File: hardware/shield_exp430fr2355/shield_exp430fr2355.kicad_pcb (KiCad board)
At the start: 2 copper layers, 74.6 x 50 mm, 50 parts, among them J1 TI_BOOSTER_40_J1, J10 Conn_01x02_Male, J12 Conn_01x02_Male, J13 Conn_01x02_Male, J14 Conn_01x02_Male, J15 Conn_01x02_Male, J16 Conn_01x02_Male, J17 Conn_01x02_Male, J18 Conn_01x02_Male, J19 Conn_01x02_Male, J2 TI_BOOSTER_40_J2, J20 Conn_01x02_Male, J21 Conn_01x02_Male, J22 Conn_01x02_Male, J23 Conn_01x02_Male, J24 Conn_01x02_Male, J25 Conn_01x02_Male, J27 Conn_01x02_Male, J28 Conn_01x02_Male, J3 TI_BOOSTER_40_J3, J4 TI_BOOSTER_40_J4, J6 Conn_02x13_Odd_Even, J7 Conn_01x02_Male, J8 Conn_01x02_Male, J9 Conn_01x02_Male, Q1 2N7002, Q2 2N7002, U1 NCP1117-3.3_SOT223

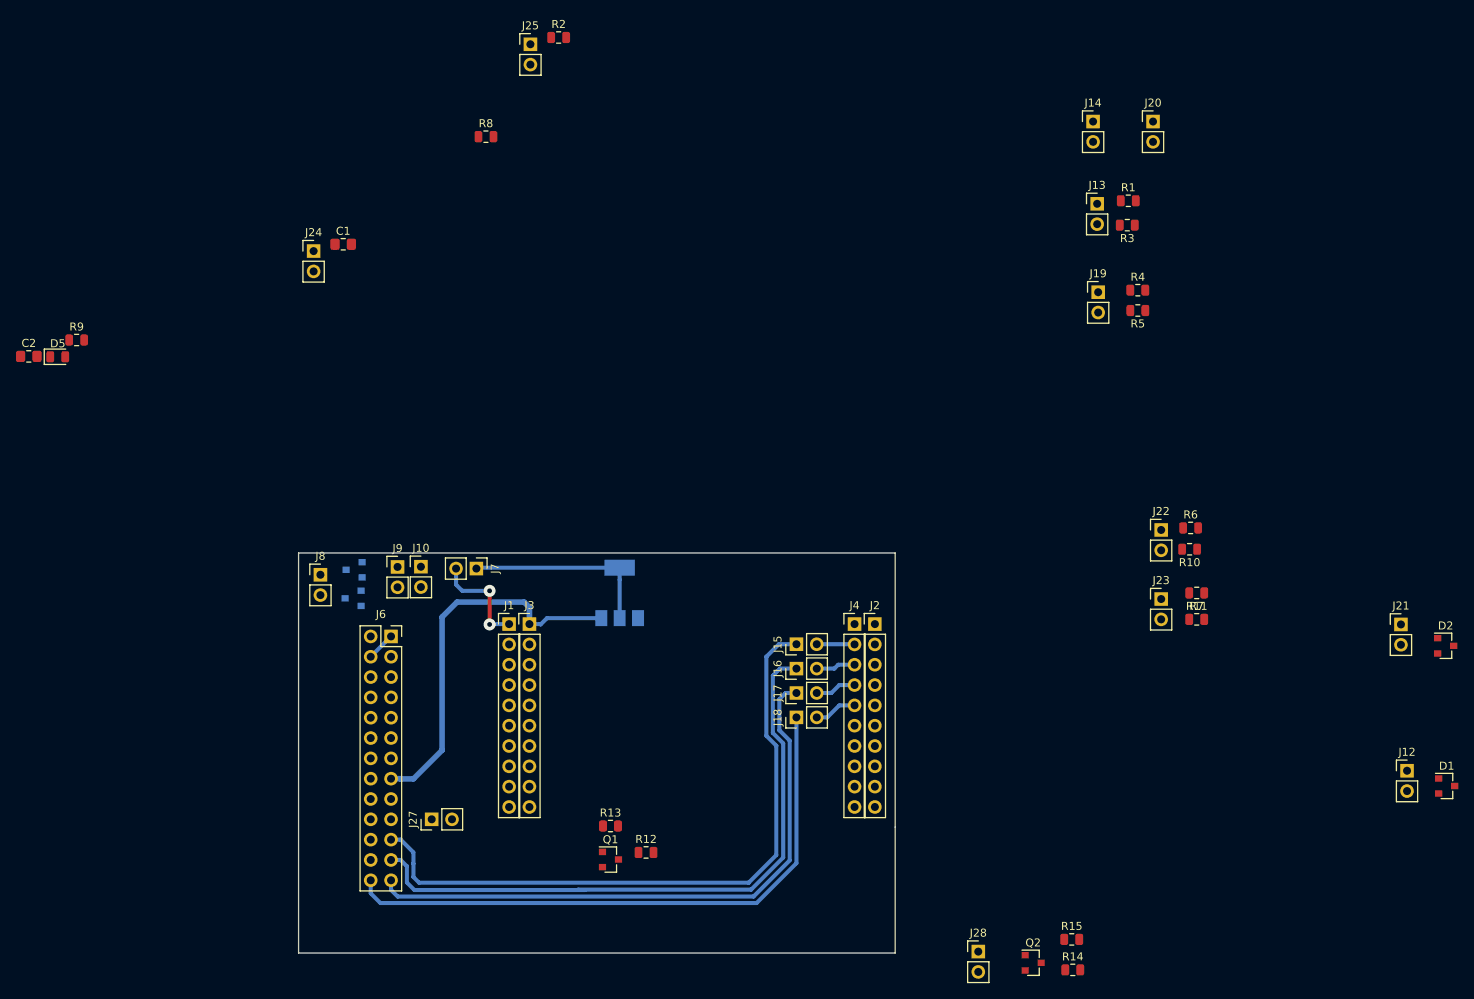
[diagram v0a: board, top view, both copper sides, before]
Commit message: Routing tracks
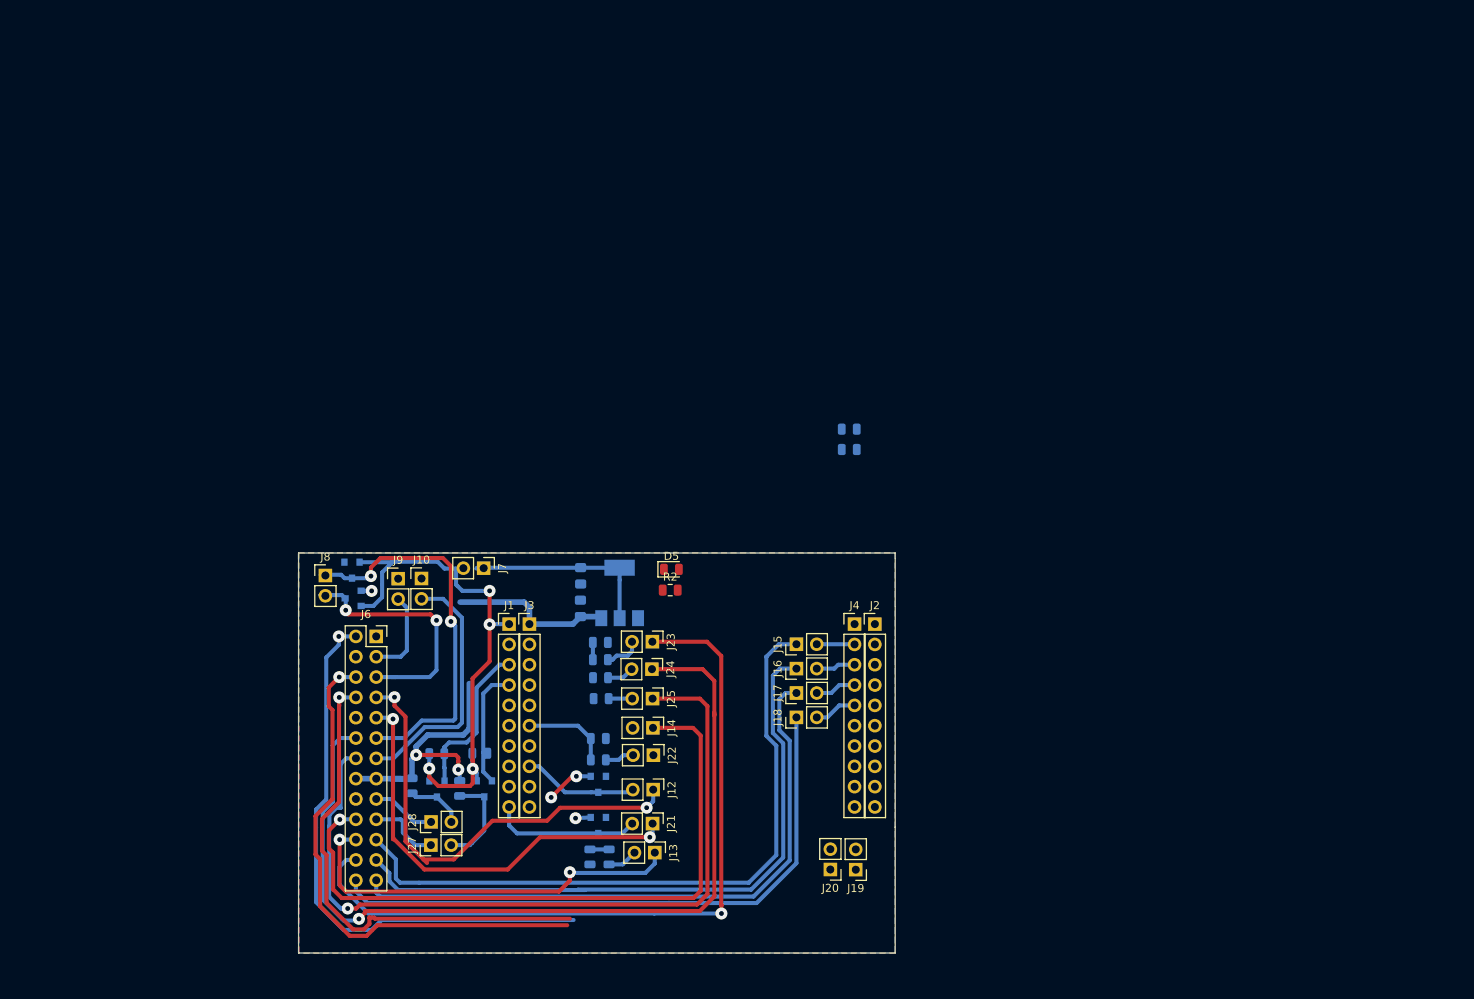
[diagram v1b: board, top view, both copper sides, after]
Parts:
- C1, C2, D1, D2, Q1, Q2, R1, R10, R11, R12, R13, R14, R15, R3, R4, R5, R6, R7, R8, R9: moved to B.Cu
- moved D2 108.3 mm to (208.5, 156.9), turned to 270 degrees
- moved D1 106.0 mm to (208.5, 151.8), turned to 270 degrees
- moved R1 104.6 mm to (209.9, 160.9), turned to 90 degrees
- moved R3 103.7 mm to (207.5, 160.9), turned to 270 degrees
- moved J20 101.8 mm to (237.5, 162.5), turned to 180 degrees
- moved J13 98.2 mm to (215.6, 160.4), turned to 270 degrees
- moved J21 96.8 mm to (215.3, 156.7), turned to 270 degrees
- moved J12 94.3 mm to (215.4, 152.5), turned to 270 degrees
- moved J14 93.7 mm to (215.4, 144.8), turned to 270 degrees
- moved R15 84.7 mm to (185.2, 152.0), turned to 270 degrees
- moved R14 84.0 mm to (188.3, 148.0)
- moved J25 83.2 mm to (215.3, 141.1), turned to 270 degrees
- moved D5 81.2 mm to (217.7, 124.9)
- moved R6 79.5 mm to (208.5, 148.8), turned to 180 degrees
- moved R9 79.4 mm to (208.9, 141.1), turned to 180 degrees
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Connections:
- J20 pad 2: P2.3 -> P2.4
- J6 pad 18: GND -> Net-(J6-Pad18)
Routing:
- net R_TCRT: track 0.00 -> 110.1 mm, vias 0 -> 1
- net L_TCRT: track 0.00 -> 99.1 mm, vias 0 -> 1
- net D1: track 0.00 -> 95.4 mm, vias 0 -> 1
- net Trig0: track 0.00 -> 84.3 mm, vias 0 -> 1
- net D0: track 0.00 -> 70.8 mm, vias 0 -> 1
- net Echo1: track 0.00 -> 65.6 mm, vias 0 -> 1
- net Trig1: track 0.00 -> 61.8 mm, vias 0 -> 1
- net ADC0: track 0.00 -> 57.9 mm, vias 0 -> 2
- net +3V3: track 13.2 -> 68.6 mm, vias 2 -> 4
- net ADC1: track 0.00 -> 54.4 mm, vias 0 -> 2
- net Echo0: track 0.00 -> 51.0 mm, vias 0 -> 2
- net ADC2: track 0.00 -> 48.8 mm, vias 0 -> 2
- net ADC3: track 0.00 -> 32.9 mm, vias 0 -> 2
- net AMP2: track 0.00 -> 31.7 mm
- net P1.6: track 0.00 -> 19.9 mm
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- added copper zone on B.Cu, net GND
- added copper zone on F.Cu, net GND
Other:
- net class +5V added: clearance 0.3048, trace_width 0.7, via_dia 1.5, via_drill 0.6
